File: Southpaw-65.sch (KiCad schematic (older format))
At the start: 88 parts

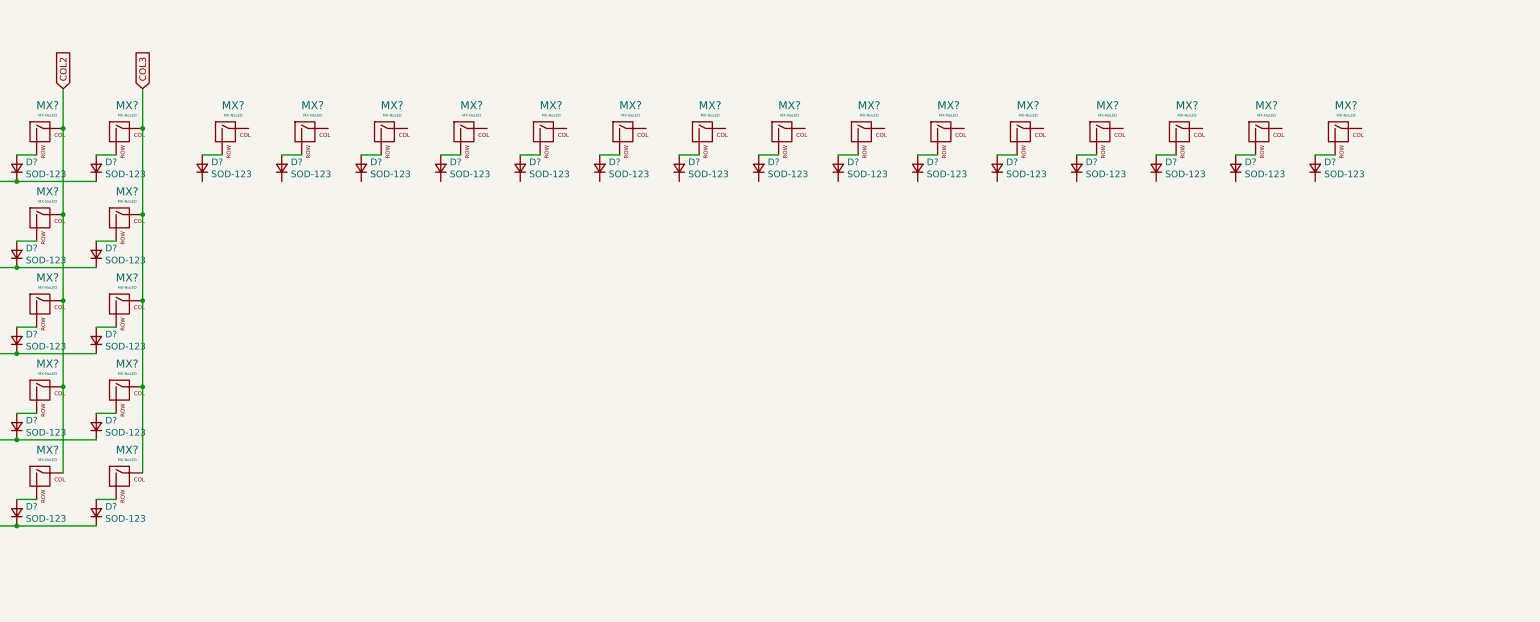
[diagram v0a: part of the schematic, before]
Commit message: Finished switch matrix
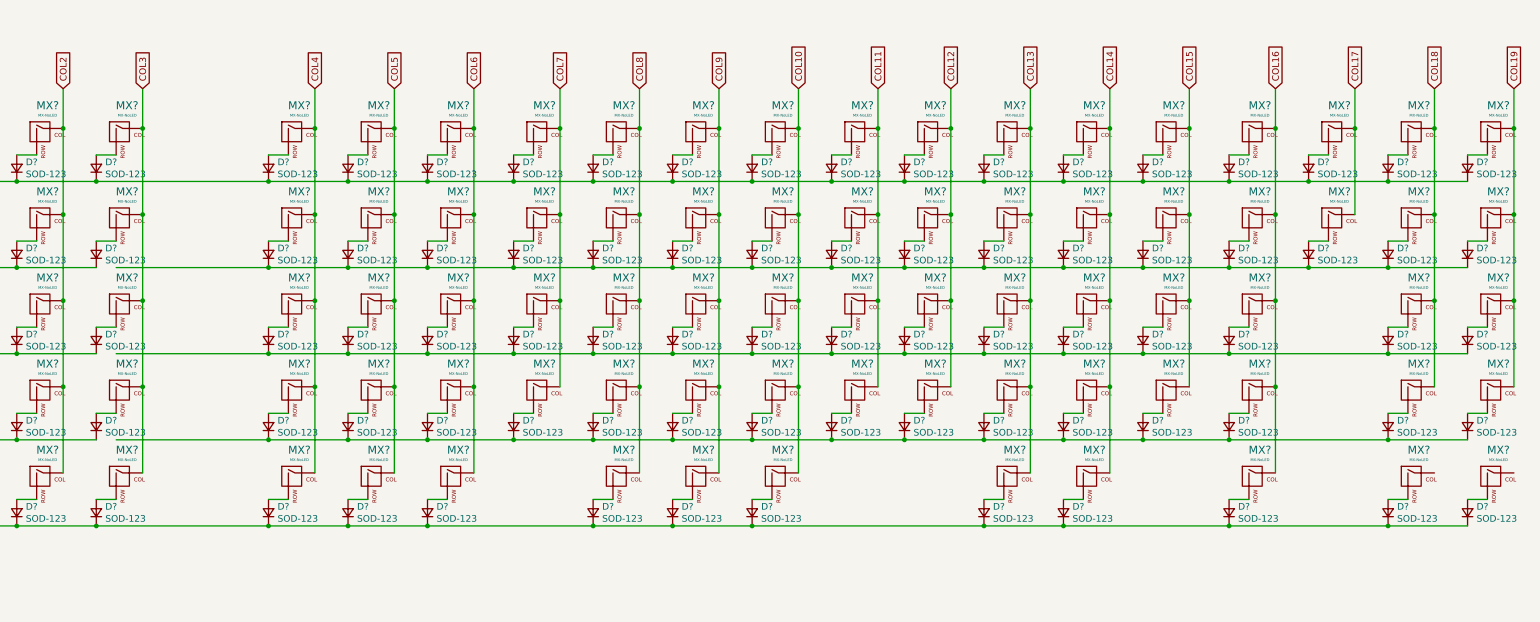
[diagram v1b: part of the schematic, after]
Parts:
- removed D?: SOD-123, symbol Device:D_Small
- removed MX?: MX-NoLED, symbol MX_Alps_Hybrid:MX-NoLED
- added D? (x59): SOD-123, symbol Device:D_Small
- added MX? (x59): MX-NoLED, symbol MX_Alps_Hybrid:MX-NoLED
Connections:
- net ROW0: now also D?.1 (K), D?.1 (K), D?.1 (K), D?.1 (K), D?.1 (K), D?.1 (K), D?.1 (K), D?.1 (K), D?.1 (K), D?.1 (K), D?.1 (K), D?.1 (K), D?.1 (K), D?.1 (K), D?.1 (K), D?.1 (K)
- net ROW4: now also D?.1 (K), D?.1 (K), D?.1 (K), D?.1 (K), D?.1 (K), D?.1 (K), D?.1 (K), D?.1 (K), D?.1 (K), D?.1 (K), D?.1 (K)
- net COL4: now reaches MX?.1 (COL)
- net COL4: now also MX?.1 (COL), MX?.1 (COL), MX?.1 (COL), MX?.1 (COL)
- net COL5: now reaches MX?.1 (COL)
- net COL5: now also MX?.1 (COL), MX?.1 (COL), MX?.1 (COL), MX?.1 (COL)
- net COL6: now reaches MX?.1 (COL)
- net COL6: now also MX?.1 (COL), MX?.1 (COL), MX?.1 (COL), MX?.1 (COL)
- net COL7: now reaches MX?.1 (COL)
- net COL7: now also MX?.1 (COL), MX?.1 (COL), MX?.1 (COL)
- net COL8: now reaches MX?.1 (COL)
- net COL8: now also MX?.1 (COL), MX?.1 (COL), MX?.1 (COL), MX?.1 (COL)
- net COL9: now reaches MX?.1 (COL)
- net COL9: now also MX?.1 (COL), MX?.1 (COL), MX?.1 (COL), MX?.1 (COL)
- net COL10: now reaches MX?.1 (COL)
- net COL10: now also MX?.1 (COL), MX?.1 (COL), MX?.1 (COL), MX?.1 (COL)
- net COL11: now reaches MX?.1 (COL)
- net COL11: now also MX?.1 (COL), MX?.1 (COL), MX?.1 (COL)
- net COL12: now reaches MX?.1 (COL)
- net COL12: now also MX?.1 (COL), MX?.1 (COL), MX?.1 (COL)
- net COL13: now reaches MX?.1 (COL)
- net COL13: now also MX?.1 (COL), MX?.1 (COL), MX?.1 (COL), MX?.1 (COL)
- net COL14: now reaches MX?.1 (COL)
- net COL14: now also MX?.1 (COL), MX?.1 (COL), MX?.1 (COL), MX?.1 (COL)
- net COL15: now reaches MX?.1 (COL)
- net COL15: now also MX?.1 (COL), MX?.1 (COL), MX?.1 (COL)
- net COL17: now reaches MX?.1 (COL)
- net COL17: now also MX?.1 (COL)
- net COL18: now reaches MX?.1 (COL)
- net COL18: now also MX?.1 (COL), MX?.1 (COL), MX?.1 (COL)
- new net: D?.2 (A), MX?.2 (ROW) (x59)
- new net: D?.1 (K), D?.1 (K), D?.1 (K), D?.1 (K), D?.1 (K), D?.1 (K), D?.1 (K), D?.1 (K), D?.1 (K), D?.1 (K), D?.1 (K), D?.1 (K), D?.1 (K), D?.1 (K), D?.1 (K), D?.1 (K)
- new net: D?.1 (K), D?.1 (K), D?.1 (K), D?.1 (K), D?.1 (K), D?.1 (K), D?.1 (K), D?.1 (K), D?.1 (K), D?.1 (K), D?.1 (K), D?.1 (K), D?.1 (K), D?.1 (K), D?.1 (K) (x2)
- new net COL16: MX?.1 (COL), MX?.1 (COL), MX?.1 (COL), MX?.1 (COL), MX?.1 (COL)
- new net COL19: MX?.1 (COL), MX?.1 (COL), MX?.1 (COL), MX?.1 (COL)
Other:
- moved on the sheet: D?, MX?
